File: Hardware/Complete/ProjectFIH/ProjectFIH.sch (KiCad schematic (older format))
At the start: 84 parts, among them J1 Conn_01x02_Male, J10 Payload LED, J2 Power, J3 Power LED, J4 MCU Fail LED, J5 Heater LED, J6 Heater, J7 UART, J8 AVR-ISP-10, J9 Payload, Q1 2N7002, Q2 2N7002, Q3 IRLZ44N, U1 74HC04, U2 74HC08, U3 74HC02, U4 LM158, U5 74HC4017, U6 LM22675-5.0, U7 LM2576S-ADJ, U8 ATmega8A-AU, Y1 8MHz

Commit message: More tracing
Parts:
- Q3: footprint Package_TO_SOT_THT:TO-220-3_Vertical -> Package_TO_SOT_THT:TO-220-3_Horizontal_TabDown
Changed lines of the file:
@@
 F 0 "Q3" H 8304 2896 50  0000 L CNN
 F 1 "IRLZ44N" H 8304 2805 50  0000 L CNN
-F 2 "Package_TO_SOT_THT:TO-220-3_Vertical" H 8350 2775 50  0001 L CIN
+F 2 "Package_TO_SOT_THT:TO-220-3_Horizontal_TabDown" H 8350 2775 50  0001 L CIN
 F 3 "http://www.irf.com/product-info/datasheets/data/irlz44n.pdf" H 8100 2850 50  0001 L CNN
 	1    8100 2850

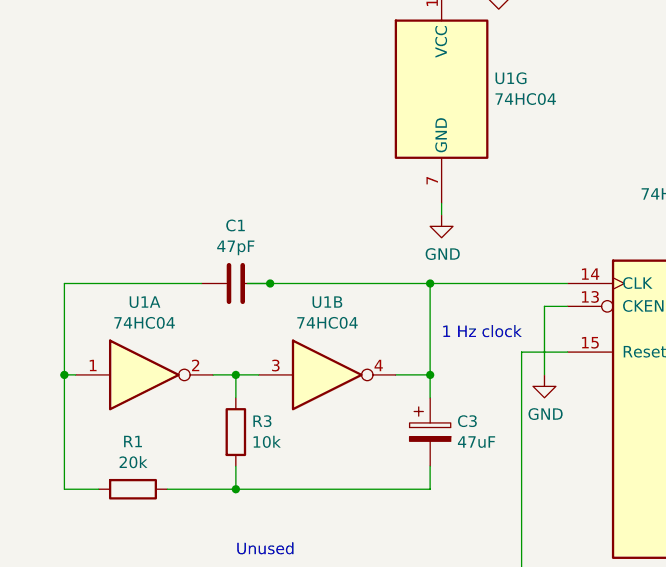
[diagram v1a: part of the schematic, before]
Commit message: More tracing
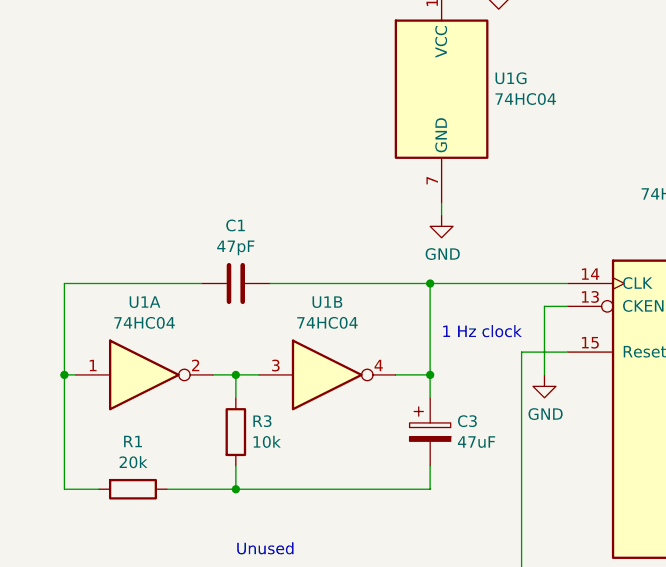
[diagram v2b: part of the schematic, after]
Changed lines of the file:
@@
 Wire Wire Line
 	8350 7150 8300 7150
-Connection ~ 1650 6200
-Wire Wire Line
-	1650 6200 1550 6200
 Wire Wire Line
 	2750 6500 2950 6500
